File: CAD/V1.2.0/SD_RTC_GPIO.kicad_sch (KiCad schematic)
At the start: 23 parts, among them K10 CR2032_BS-6-1, K11 HYC77-TF09-200, Q14 PMOS, SW3 K2-1114SA-A4SW-06, U7 PCF85063A, X1 7LC32768F12UC

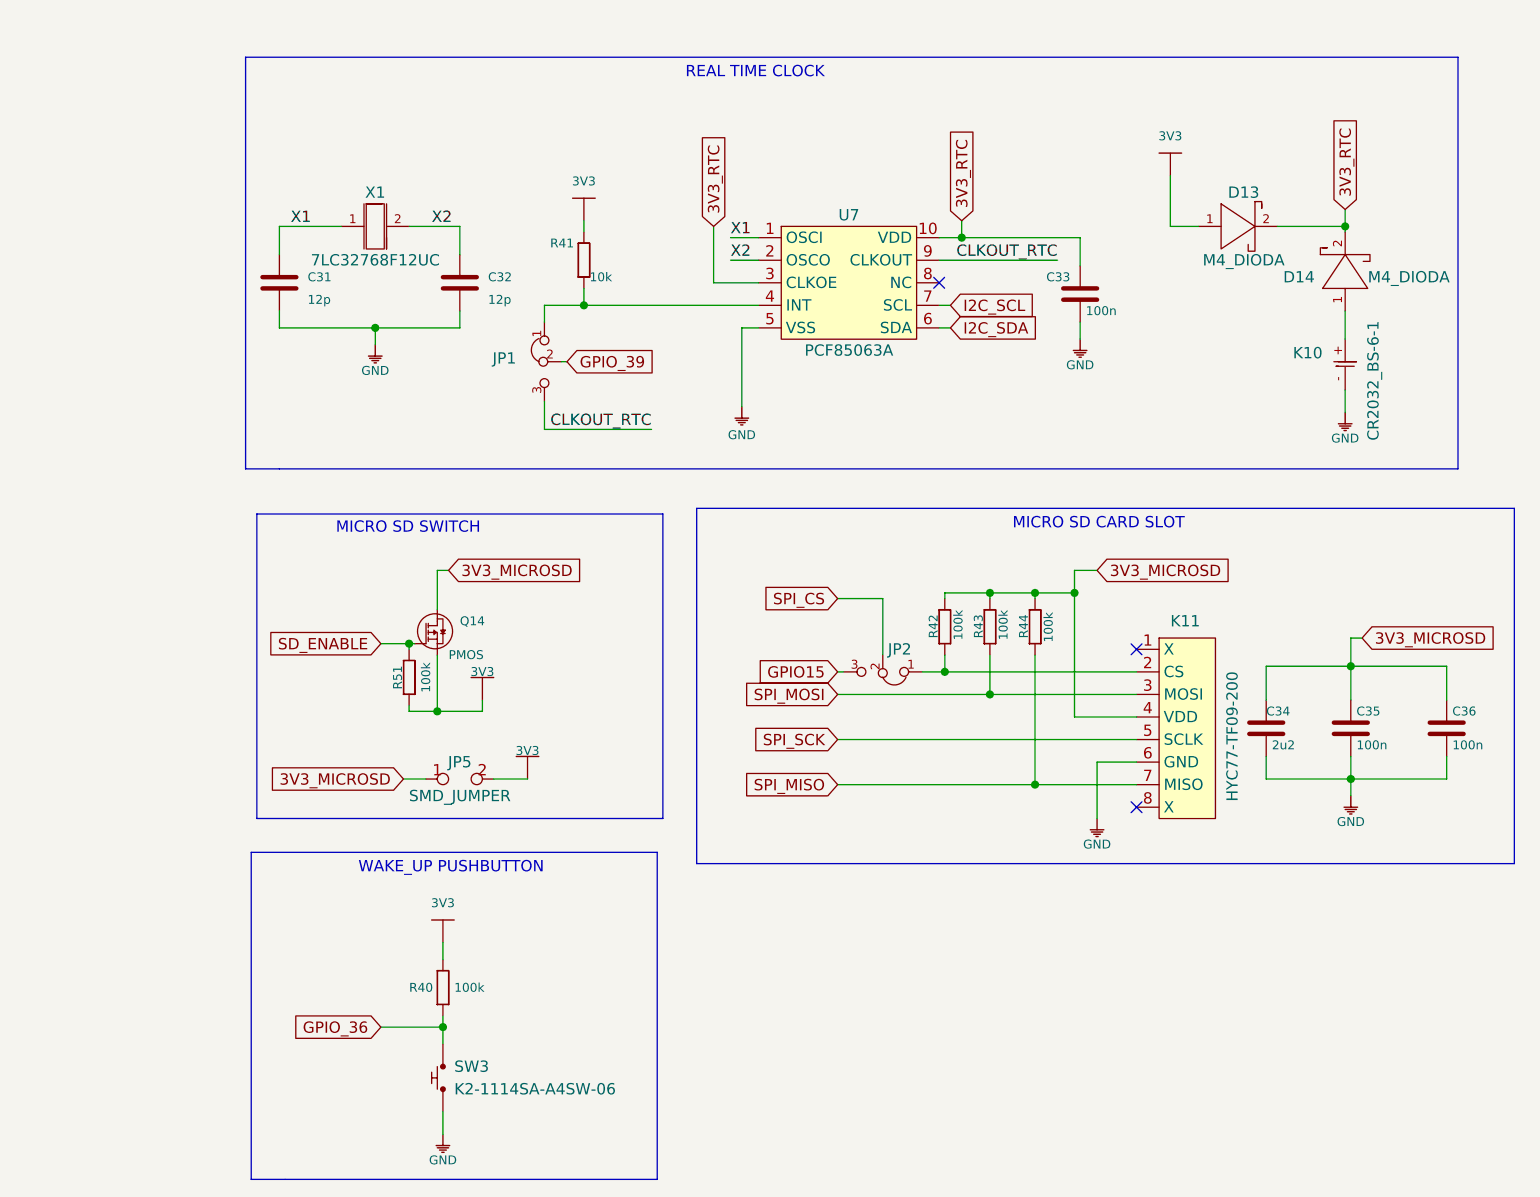
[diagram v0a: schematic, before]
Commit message: Updating open source files.
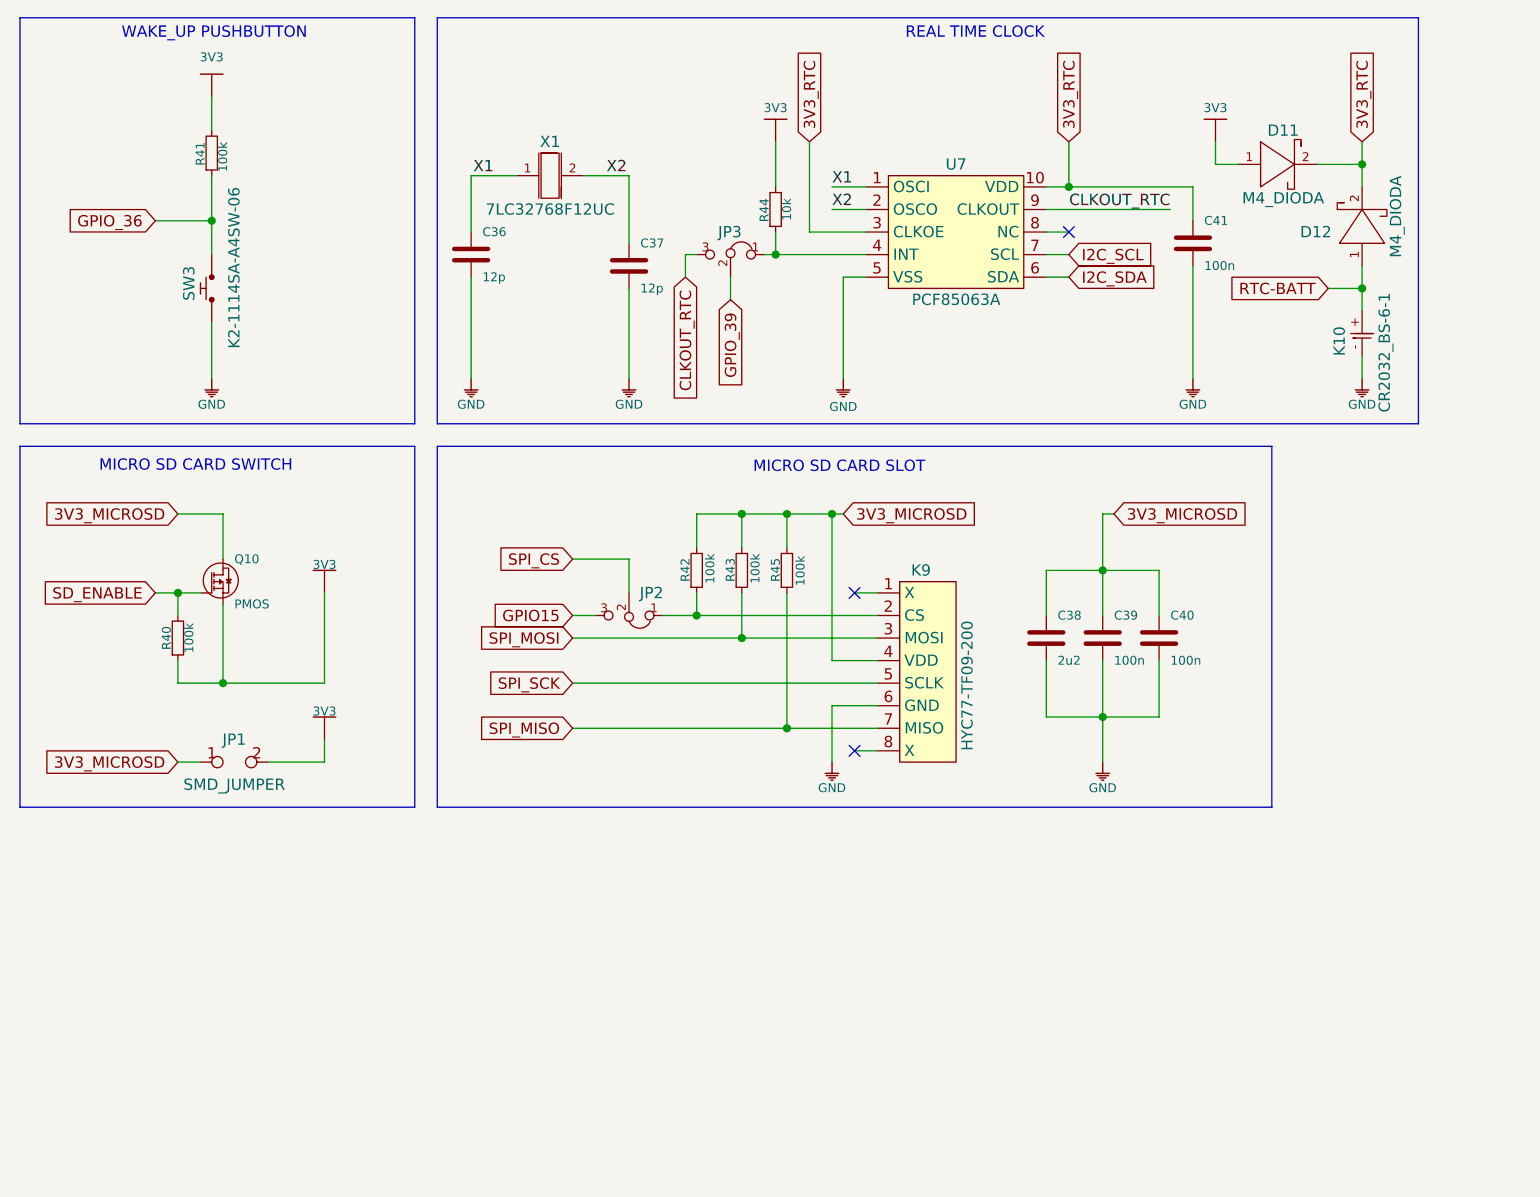
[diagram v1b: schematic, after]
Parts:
- renumbered C31 to C36, C32 to C37, C34 to C38, C35 to C39, C36 to C40, C33 to C41, D13 to D11, D14 to D12, JP5 to JP1, JP1 to JP3, K11 to K9, Q14 to Q10, R51 to R40, R40 to R41, R41 to R44, R44 to R45
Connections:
- net RTC-BATT: now reaches D12.1 (A), K10.+
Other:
- note added: "MICRO SD CARD SWITCH"
- note removed: "MICRO SD SWITCH"
- title: Soldered Inkplate 6PLUS -> Soldered Inkplate 6 FLICK
- moved on the sheet: C36, C37, C38, C39, C40, C41, D11, D12, JP1, JP2, JP3, K10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
